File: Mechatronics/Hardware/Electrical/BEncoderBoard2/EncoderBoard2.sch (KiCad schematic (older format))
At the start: 43 parts, among them J1 Conn_01x08_Male, J2 Conn_01x07_Male, J6 Conn_01x04_Male, Q3 Q_PMOS_GSD, U1 STM32G431CBT6, U2 ITR1802, U3 ITR1802, U4 RN4871, Y1 8Mhz

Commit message: Changes
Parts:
- U2, U3: value ITR1802 -> ITR1802_Conn; footprint Encoder:OptointerrupterSmall -> Encoder:PinHeader_2x02_P2.54mm_Vertical
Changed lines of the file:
@@
 P 1500 1950
 F 0 "U2" H 1500 2275 50  0000 C CNN
-F 1 "ITR1802" H 1500 2184 50  0000 C CNN
-F 2 "Encoder:OptointerrupterSmall" H 1500 1950 50  0001 C CNN
+F 1 "ITR1802_Conn" H 1500 2184 50  0000 C CNN
+F 2 "Encoder:PinHeader_2x02_P2.54mm_Vertical" H 1500 1950 50  0001 C CNN
 F 3 "" H 1500 1950 50  0001 C CNN
 	1    1500 1950
@@
 P 1500 2850
 F 0 "U3" H 1500 3175 50  0000 C CNN
-F 1 "ITR1802" H 1500 3084 50  0000 C CNN
-F 2 "Encoder:OptointerrupterSmall" H 1500 2850 50  0001 C CNN
+F 1 "ITR1802_Conn" H 1500 2650 50  0000 C CNN
+F 2 "Encoder:PinHeader_2x02_P2.54mm_Vertical" H 1500 2850 50  0001 C CNN
 F 3 "" H 1500 2850 50  0001 C CNN
 	1    1500 2850

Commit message: Changed name
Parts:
- removed U2, U3: ITR1802_Conn, Encoder:PinHeader_2x02_P2.54mm_Vertical, symbol Encoder:ITR1802
- added U2, U3: ITR8102_Conn, Encoder:PinHeader_2x02_P2.54mm_Vertical, symbol Encoder:ITR8102
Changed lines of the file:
@@
 Comment4 ""
 $EndDescr
-$Comp
-L Encoder:ITR1802 U2
-U 1 1 5C28311C
-P 1500 1950
-F 0 "U2" H 1500 2275 50  0000 C CNN
-F 1 "ITR1802_Conn" H 1500 2184 50  0000 C CNN
-F 2 "Encoder:PinHeader_2x02_P2.54mm_Vertical" H 1500 1950 50  0001 C CNN
-F 3 "" H 1500 1950 50  0001 C CNN
-	1    1500 1950
-	1    0    0    -1
-$EndComp
-$Comp
-L Encoder:ITR1802 U3
-U 1 1 5C28324D
-P 1500 2850
-F 0 "U3" H 1500 3175 50  0000 C CNN
-F 1 "ITR1802_Conn" H 1500 2650 50  0000 C CNN
-F 2 "Encoder:PinHeader_2x02_P2.54mm_Vertical" H 1500 2850 50  0001 C CNN
-F 3 "" H 1500 2850 50  0001 C CNN
-	1    1500 2850
-	1    0    0    -1
-$EndComp
 Wire Wire Line
 	1200 2050 1200 2100
@@
 Wire Wire Line
 	4900 900  5450 900
+$Comp
+L Encoder:ITR8102 U3
+U 1 1 5F14F36F
+P 1500 2850
+F 0 "U3" H 1500 3100 50  0000 C CNN
+F 1 "ITR8102_Conn" H 1500 2650 50  0000 C CNN
+F 2 "Encoder:PinHeader_2x02_P2.54mm_Vertical" H 1500 2850 50  0001 C CNN
+F 3 "" H 1500 2850 50  0001 C CNN
+	1    1500 2850
+	1    0    0    -1
+$EndComp
+$Comp
+L Encoder:ITR8102 U2
+U 1 1 5F152A91
+P 1500 1950
+F 0 "U2" H 1500 2250 50  0000 C CNN
+F 1 "ITR8102_Conn" H 1500 2150 50  0000 C CNN
+F 2 "Encoder:PinHeader_2x02_P2.54mm_Vertical" H 1500 1950 50  0001 C CNN
+F 3 "" H 1500 1950 50  0001 C CNN
+	1    1500 1950
+	1    0    0    -1
+$EndComp
 $EndSCHEMATC

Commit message: Changed files
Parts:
- removed U2, U3: ITR8102_Conn, Encoder:PinHeader_2x02_P2.54mm_Vertical, symbol Encoder:ITR8102
- added U2, U3: OPTO_Conn, Encoder:PinHeader_2x02_P2.54mm_Vertical, symbol Encoder:OPTO_Conn
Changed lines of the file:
@@
 	4900 900  5450 900
 $Comp
-L Encoder:ITR8102 U3
-U 1 1 5F14F36F
+L Encoder:OPTO_Conn U3
+U 1 1 5F1557B4
 P 1500 2850
-F 0 "U3" H 1500 3100 50  0000 C CNN
-F 1 "ITR8102_Conn" H 1500 2650 50  0000 C CNN
+F 0 "U3" H 1500 3175 50  0000 C CNN
+F 1 "OPTO_Conn" H 1500 3084 50  0000 C CNN
 F 2 "Encoder:PinHeader_2x02_P2.54mm_Vertical" H 1500 2850 50  0001 C CNN
 F 3 "" H 1500 2850 50  0001 C CNN
@@
 $EndComp
 $Comp
-L Encoder:ITR8102 U2
-U 1 1 5F152A91
+L Encoder:OPTO_Conn U2
+U 1 1 5F15DEA7
 P 1500 1950
-F 0 "U2" H 1500 2250 50  0000 C CNN
-F 1 "ITR8102_Conn" H 1500 2150 50  0000 C CNN
+F 0 "U2" H 1500 2275 50  0000 C CNN
+F 1 "OPTO_Conn" H 1500 2184 50  0000 C CNN
 F 2 "Encoder:PinHeader_2x02_P2.54mm_Vertical" H 1500 1950 50  0001 C CNN
 F 3 "" H 1500 1950 50  0001 C CNN

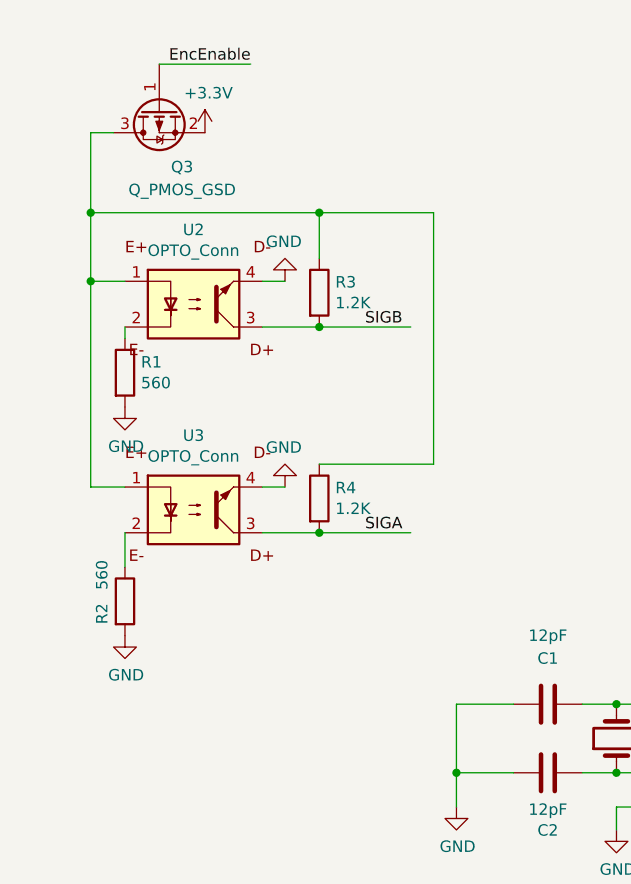
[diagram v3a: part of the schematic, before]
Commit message: Changed files
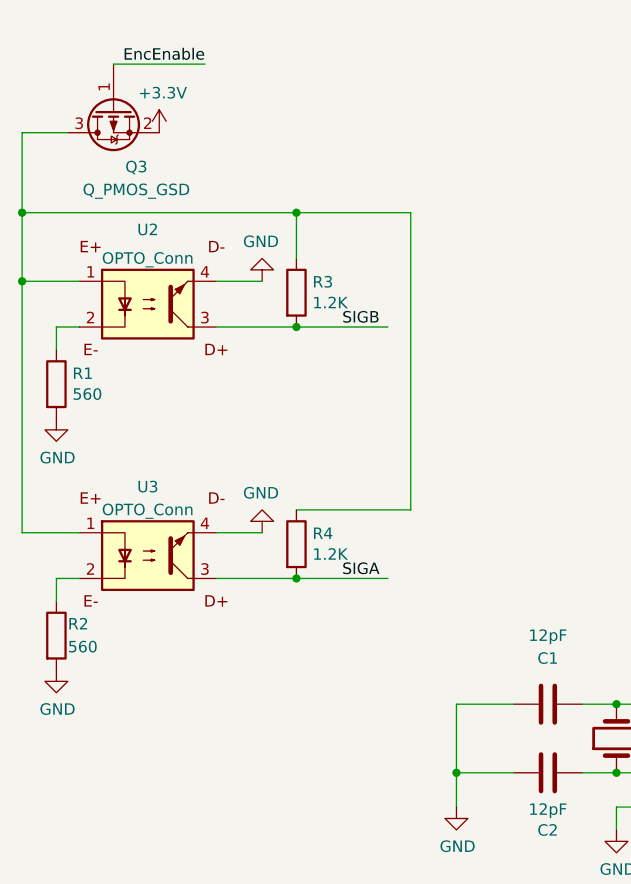
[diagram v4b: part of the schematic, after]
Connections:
- wire segments 116 -> 118
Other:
- moved on the sheet: Q3, R1, R2, R3, R4, U2, U3
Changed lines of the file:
@@
 Comment4 ""
 $EndDescr
-Wire Wire Line
-	1200 2050 1200 2100
 $Comp
 L Device:R R1
 U 1 1 5C285A10
-P 1200 2250
-F 0 "R1" H 1270 2296 50  0000 L CNN
-F 1 "560" H 1270 2205 50  0000 L CNN
-F 2 "Encoder:R_0603_1608Metric_Pad1.05x0.95mm_HandSolder" V 1130 2250 50  0001 C CNN
-F 3 "~" H 1200 2250 50  0001 C CNN
-	1    1200 2250
+P 900 2300
+F 0 "R1" H 970 2346 50  0000 L CNN
+F 1 "560" H 970 2255 50  0000 L CNN
+F 2 "Encoder:R_0603_1608Metric_Pad1.05x0.95mm_HandSolder" V 830 2300 50  0001 C CNN
+F 3 "~" H 900 2300 50  0001 C CNN
+	1    900  2300
 	1    0    0    -1
 $EndComp
@@
 L Device:R R2
 U 1 1 5C285A71
-P 1200 3250
-F 0 "R2" V 1100 3150 50  0000 L CNN
-F 1 "560" V 1100 3300 50  0000 L CNN
-F 2 "Encoder:R_0603_1608Metric_Pad1.05x0.95mm_HandSolder" V 1130 3250 50  0001 C CNN
-F 3 "~" H 1200 3250 50  0001 C CNN
-	1    1200 3250
+P 900 3400
+F 0 "R2" H 950 3450 50  0000 L CNN
+F 1 "560" H 950 3350 50  0000 L CNN
+F 2 "Encoder:R_0603_1608Metric_Pad1.05x0.95mm_HandSolder" V 830 3400 50  0001 C CNN
+F 3 "~" H 900 3400 50  0001 C CNN
+	1    900  3400
 	1    0    0    -1
 $EndComp
@@
 L power:GND #PWR0110
 U 1 1 5C2863B3
-P 1200 2400
-F 0 "#PWR0110" H 1200 2150 50  0001 C CNN
-F 1 "GND" H 1205 2227 50  0000 C CNN
-F 2 "" H 1200 2400 50  0001 C CNN
-F 3 "" H 1200 2400 50  0001 C CNN
-	1    1200 2400
+P 900 2450
+F 0 "#PWR0110" H 900 2200 50  0001 C CNN
+F 1 "GND" H 905 2277 50  0000 C CNN
+F 2 "" H 900 2450 50  0001 C CNN
+F 3 "" H 900 2450 50  0001 C CNN
+	1    900  2450
 	1    0    0    -1
 $EndComp
@@
 L power:GND #PWR0112
 U 1 1 5C2895D3
-P 1900 1850
-F 0 "#PWR0112" H 1900 1600 50  0001 C CNN
-F 1 "GND" H 1905 1677 50  0000 C CNN
-F 2 "" H 1900 1850 50  0001 C CNN
-F 3 "" H 1900 1850 50  0001 C CNN
-	1    1900 1850
+P 1800 1850
+F 0 "#PWR0112" H 1800 1600 50  0001 C CNN
+F 1 "GND" H 1805 1677 50  0000 C CNN
+F 2 "" H 1800 1850 50  0001 C CNN
+F 3 "" H 1800 1850 50  0001 C CNN
+	1    1800 1850
 	-1   0    0    1
 $EndComp
@@
 L power:GND #PWR0113
 U 1 1 5C289611
-P 1900 2750
-F 0 "#PWR0113" H 1900 2500 50  0001 C CNN
-F 1 "GND" H 1905 2577 50  0000 C CNN
-F 2 "" H 1900 2750 50  0001 C CNN
-F 3 "" H 1900 2750 50  0001 C CNN
-	1    1900 2750
-	-1   0    0    1
-$EndComp
-Wire Wire Line
-	1800 1850 1900 1850
-Wire Wire Line
-	1900 2750 1800 2750
+P 1800 2950
+F 0 "#PWR0113" H 1800 2700 50  0001 C CNN
+F 1 "GND" H 1805 2777 50  0000 C CNN
+F 2 "" H 1800 2950 50  0001 C CNN
+F 3 "" H 1800 2950 50  0001 C CNN
+	1    1800 2950
+	-1   0    0    1
+$EndComp
+Wire Wire Line
+	1600 1850 1800 1850
+Wire Wire Line
+	1800 2950 1600 2950
 $Comp
 L Device:R R3
 U 1 1 5C28C76B
-P 2050 1900
-F 0 "R3" H 2120 1946 50  0000 L CNN
-F 1 "1.2K" H 2120 1855 50  0000 L CNN
-F 2 "Encoder:R_0603_1608Metric_Pad1.05x0.95mm_HandSolder" V 1980 1900 50  0001 C CNN
-F 3 "~" H 2050 1900 50  0001 C CNN
-	1    2050 1900
-	1    0    0    -1
-$EndComp
-Text Label 2250 2050 0    50   ~ 0
+P 1950 1900
+F 0 "R3" H 2020 1946 50  0000 L CNN
+F 1 "1.2K" H 2020 1855 50  0000 L CNN
+F 2 "Encoder:R_0603_1608Metric_Pad1.05x0.95mm_HandSolder" V 1880 1900 50  0001 C CNN
+F 3 "~" H 1950 1900 50  0001 C CNN
+	1    1950 1900
+	1    0    0    -1
+$EndComp
+Text Label 2150 2050 0    50   ~ 0
 SIGB
 Wire Wire Line
-	1800 2050 2050 2050
-Wire Wire Line
-	2050 2050 2450 2050
-Connection ~ 2050 2050
+	1600 2050 1950 2050
+Wire Wire Line
+	1950 2050 2350 2050
+Connection ~ 1950 2050
 $Comp
 L Device:R R4
 U 1 1 5C293966
-P 2050 2800
-F 0 "R4" H 2120 2846 50  0000 L CNN
-F 1 "1.2K" H 2120 2755 50  0000 L CNN
-F 2 "Encoder:R_0603_1608Metric_Pad1.05x0.95mm_HandSolder" V 1980 2800 50  0001 C CNN
-F 3 "~" H 2050 2800 50  0001 C CNN
-	1    2050 2800
-	1    0    0    -1
-$EndComp
-Wire Wire Line
-	1800 2950 2050 2950
-Wire Wire Line
-	2050 2950 2450 2950
-Connection ~ 2050 2950
-Text Label 2250 2950 0    50   ~ 0
+P 1950 3000
+F 0 "R4" H 2020 3046 50  0000 L CNN
+F 1 "1.2K" H 2020 2955 50  0000 L CNN
+F 2 "Encoder:R_0603_1608Metric_Pad1.05x0.95mm_HandSolder" V 1880 3000 50  0001 C CNN
+F 3 "~" H 1950 3000 50  0001 C CNN
+	1    1950 3000
+	1    0    0    -1
+$EndComp
+Wire Wire Line
+	1600 3150 1950 3150
+Wire Wire Line
+	1950 3150 2350 3150
+Connection ~ 1950 3150
+Text Label 2150 3150 0    50   ~ 0
 SIGA
 $Comp
 L Encoder:Q_PMOS_GSD Q3
 U 1 1 5D553268
-P 1350 1150
-F 0 "Q3" H 1450 950 50  0000 C CNN
-F 1 "Q_PMOS_GSD" H 1450 850 50  0000 C CNN
-F 2 "Encoder:SOT-23" V 1550 1000 50  0001 C CNN
-F 3 "~" V 1350 1200 50  0001 C CNN
-	1    1350 1150
-	1    0    0    -1
-$EndComp
-Text Label 1750 900  2    50   ~ 0
+P 1150 1150
+F 0 "Q3" H 1250 950 50  0000 C CNN
+F 1 "Q_PMOS_GSD" H 1250 850 50  0000 C CNN
+F 2 "Encoder:SOT-23" V 1350 1000 50  0001 C CNN
+F 3 "~" V 1150 1200 50  0001 C CNN
+	1    1150 1150
+	1    0    0    -1
+$EndComp
+Text Label 1550 900  2    50   ~ 0
 EncEnable
 Wire Wire Line
-	1750 900  1350 900
+	1550 900  1150 900
 $Comp
 L power:+3.3V #PWR017
 U 1 1 5D59FF5B
-P 1550 1200
-F 0 "#PWR017" H 1550 1050 50  0001 C CNN
-F 1 "+3.3V" H 1565 1373 50  0000 C CNN
-F 2 "" H 1550 1200 50  0001 C CNN
-F 3 "" H 1550 1200 50  0001 C CNN
-	1    1550 1200
-	1    0    0    -1
-$EndComp
-Wire Wire Line
-	2050 1750 2050 1550
-Wire Wire Line
-	2050 2650 2550 2650
-Wire Wire Line
-	2550 2650 2550 1550
-Wire Wire Line
-	2550 1550 2050 1550
-Connection ~ 2050 1550
-Wire Wire Line
-	1050 2750 1050 1850
-Wire Wire Line
-	1050 1200 1150 1200
-Wire Wire Line
-	1050 2750 1200 2750
-Wire Wire Line
-	1050 1550 2050 1550
-Connection ~ 1050 1550
-Wire Wire Line
-	1050 1550 1050 1200
-Wire Wire Line
-	1050 1850 1200 1850
-Connection ~ 1050 1850
-Wire Wire Line
-	1050 1850 1050 1550
+P 1350 1200
+F 0 "#PWR017" H 1350 1050 50  0001 C CNN
+F 1 "+3.3V" H 1365 1373 50  0000 C CNN
+F 2 "" H 1350 1200 50  0001 C CNN
+F 3 "" H 1350 1200 50  0001 C CNN
+	1    1350 1200
+	1    0    0    -1
+$EndComp
+Wire Wire Line
+	1950 1750 1950 1550
+Wire Wire Line
+	1950 2850 2450 2850
+Wire Wire Line
+	2450 2850 2450 1550
+Wire Wire Line
+	2450 1550 1950 1550
+Connection ~ 1950 1550
+Wire Wire Line
+	750  2950 750  1850
+Wire Wire Line
+	750  1200 950  1200
+Wire Wire Line
+	750  2950 1000 2950
+Wire Wire Line
+	750  1550 1950 1550
+Connection ~ 750  1550
+Wire Wire Line
+	750  1550 750  1200
+Wire Wire Line
+	750  1850 1000 1850
+Connection ~ 750  1850
+Wire Wire Line
+	750  1850 750  1550
 $Comp
 L Encoder:RN4871 U4
@@
 L power:GND #PWR0128
 U 1 1 5F196248
-P 1200 3400
-F 0 "#PWR0128" H 1200 3150 50  0001 C CNN
-F 1 "GND" H 1205 3227 50  0000 C CNN
-F 2 "" H 1200 3400 50  0001 C CNN
-F 3 "" H 1200 3400 50  0001 C CNN
-	1    1200 3400
-	1    0    0    -1
-$EndComp
-Wire Wire Line
-	1200 3100 1200 2950
+P 900 3550
+F 0 "#PWR0128" H 900 3300 50  0001 C CNN
+F 1 "GND" H 905 3377 50  0000 C CNN
+F 2 "" H 900 3550 50  0001 C CNN
+F 3 "" H 900 3550 50  0001 C CNN
+	1    900  3550
+	1    0    0    -1
+$EndComp
 Wire Wire Line
 	5450 1200 5100 1200
@@
 L Encoder:OPTO_Conn U3
 U 1 1 5F1557B4
-P 1500 2850
-F 0 "U3" H 1500 3175 50  0000 C CNN
-F 1 "OPTO_Conn" H 1500 3084 50  0000 C CNN
-F 2 "Encoder:PinHeader_2x02_P2.54mm_Vertical" H 1500 2850 50  0001 C CNN
-F 3 "" H 1500 2850 50  0001 C CNN
-	1    1500 2850
+P 1300 3050
+F 0 "U3" H 1300 3350 50  0000 C CNN
+F 1 "OPTO_Conn" H 1300 3250 50  0000 C CNN
+F 2 "Encoder:PinHeader_2x02_P2.54mm_Vertical" H 1300 3050 50  0001 C CNN
+F 3 "" H 1300 3050 50  0001 C CNN
+	1    1300 3050
 	1    0    0    -1
 $EndComp
@@
 L Encoder:OPTO_Conn U2
 U 1 1 5F15DEA7
-P 1500 1950
-F 0 "U2" H 1500 2275 50  0000 C CNN
-F 1 "OPTO_Conn" H 1500 2184 50  0000 C CNN
-F 2 "Encoder:PinHeader_2x02_P2.54mm_Vertical" H 1500 1950 50  0001 C CNN
-F 3 "" H 1500 1950 50  0001 C CNN
-	1    1500 1950
-	1    0    0    -1
-$EndComp
+P 1300 1950
+F 0 "U2" H 1300 2275 50  0000 C CNN
+F 1 "OPTO_Conn" H 1300 2150 50  0000 C CNN
+F 2 "Encoder:PinHeader_2x02_P2.54mm_Vertical" H 1300 1950 50  0001 C CNN
+F 3 "" H 1300 1950 50  0001 C CNN
+	1    1300 1950
+	1    0    0    -1
+$EndComp
+Wire Wire Line
+	900  2150 900  2050
+Wire Wire Line
+	900  2050 1000 2050
+Wire Wire Line
+	900  3250 900  3150
+Wire Wire Line
+	900  3150 1000 3150
 $EndSCHEMATC
